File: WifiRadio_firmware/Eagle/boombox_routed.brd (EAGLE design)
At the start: 65.7 x 50.8 mm, 16 parts, among them Y1 16 MHz

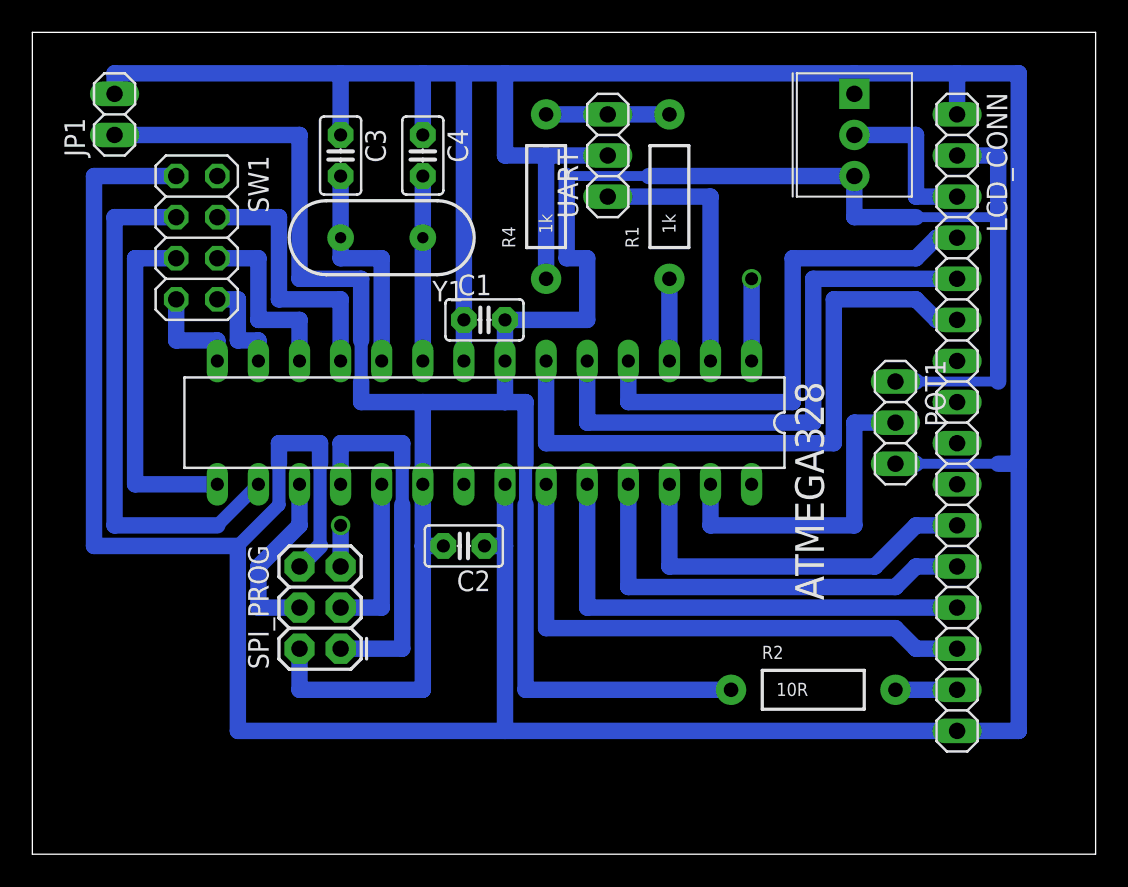
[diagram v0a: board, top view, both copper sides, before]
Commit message: Finished manual routing
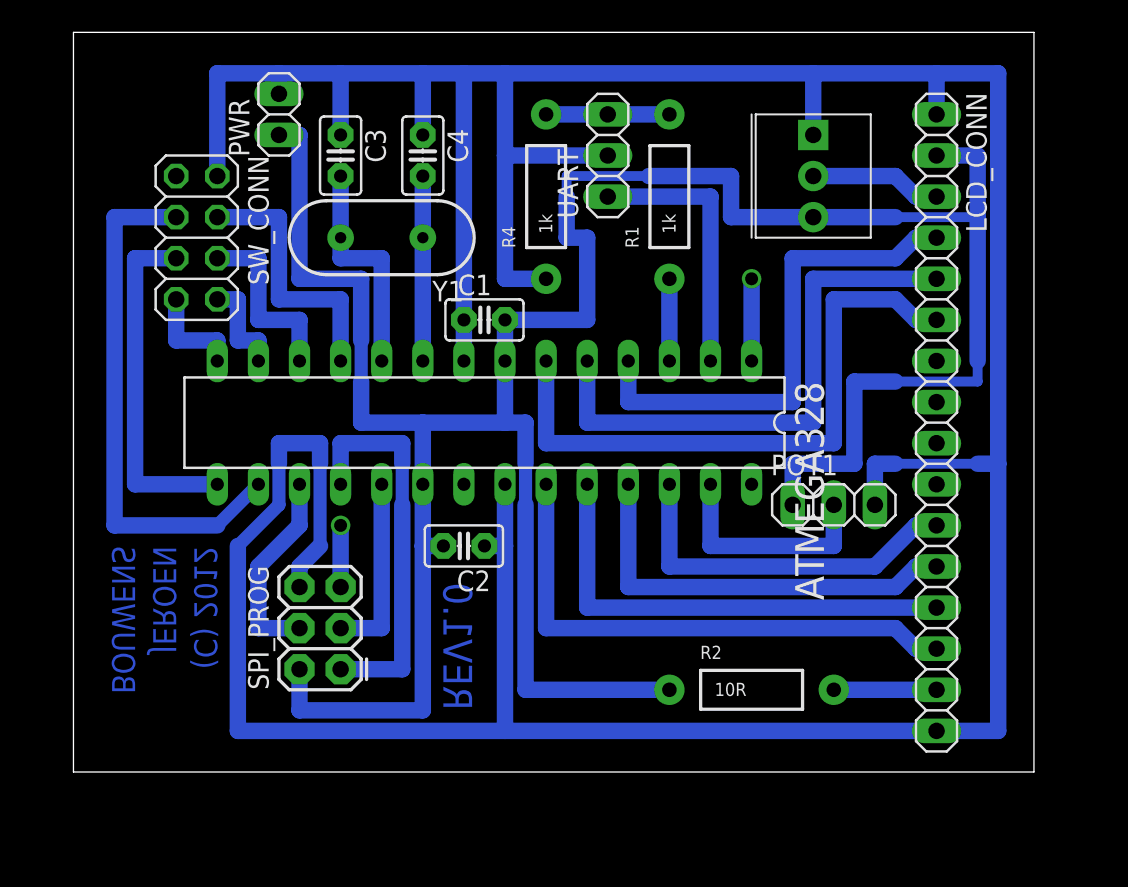
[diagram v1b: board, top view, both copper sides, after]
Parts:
- removed JP1: (no value), pinhead:1X02
- added PWR: (no value), pinhead:1X02
- moved POT1 6.35 mm to (49.5, 17.8), turned to 0 degrees
- moved R2 3.81 mm to (44.5, 6.35)
- moved CONTR 3.59 mm to (45.7, 40.6)
- moved SPI_PROG 1.27 mm to (19.1, 7.62)
- moved LCD_CONN 1.27 mm to (55.9, 22.9)
- renumbered SW1 to SW_CONN
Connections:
- net GND: now also PWR.2, SW_CONN.2; no longer JP1.2, SW_CONN.1
- net VCC: now also PWR.1; no longer JP1.1
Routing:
- net GND: track 284.8 -> 254.3 mm
- net N$20: track 20.3 -> 14.0 mm
- net N$10: track 3.81 -> 6.35 mm
- net N$3: track 10.2 -> 8.15 mm
- net N$27: track 7.62 -> 8.89 mm
- net N$18: track 11.2 -> 12.5 mm
- net N$17: track 22.9 -> 24.1 mm
- net N$16: track 10.2 -> 11.4 mm
- net N$9: track 39.9 -> 38.6 mm
- net N$8: track 35.6 -> 34.3 mm
- net N$14: track 23.9 -> 22.6 mm
- net N$13: track 27.2 -> 25.9 mm
- net N$12: track 30.5 -> 29.2 mm
- net N$11: track 34.8 -> 33.5 mm
- net N$7: track 32.3 -> 31.0 mm
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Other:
- board size 65.7 x 50.8 mm -> 59.4 x 45.7 mm
- board text added: "(C) 2012"
- board text added: "BOUWENS"
- board text added: "JEROEN"
- board text added: "REV1.0"
